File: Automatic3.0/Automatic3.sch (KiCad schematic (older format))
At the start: 56 parts, among them J1 GND VCC, J10 Line Tracker and Proximity, J11 Compass, J12 Bluetooth, J13 Encoder, J14 Bluetooth, J15 Motor, J19 Bluetooth, J2 CONN_01X01, J4 CONN_01X01, J5 CONN_01X01, J6 I/O Pins, J7 USB_B, J8 CONN_01X01, J9 I/O Pins, U1 Arduino_Mega2560_Shield, U2 Arduino_Mega2560_Shield

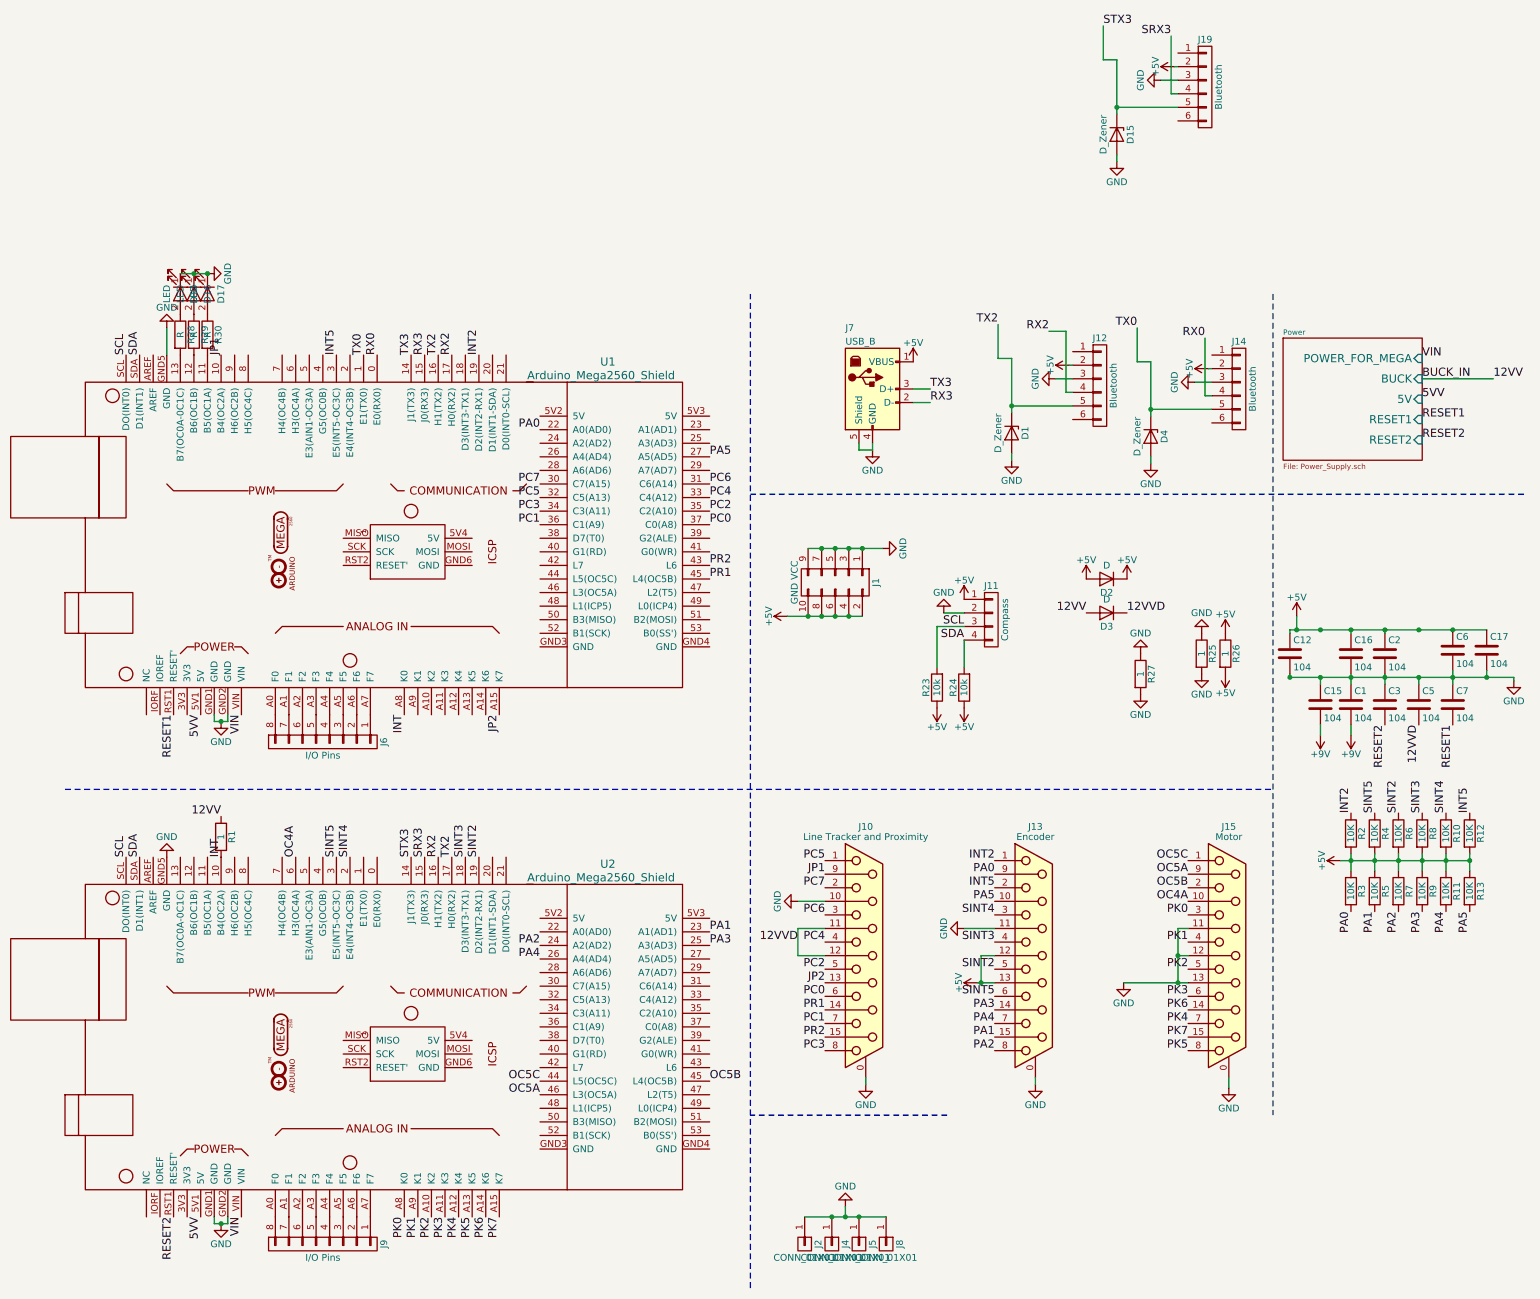
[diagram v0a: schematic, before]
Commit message: modified the automatic circuit
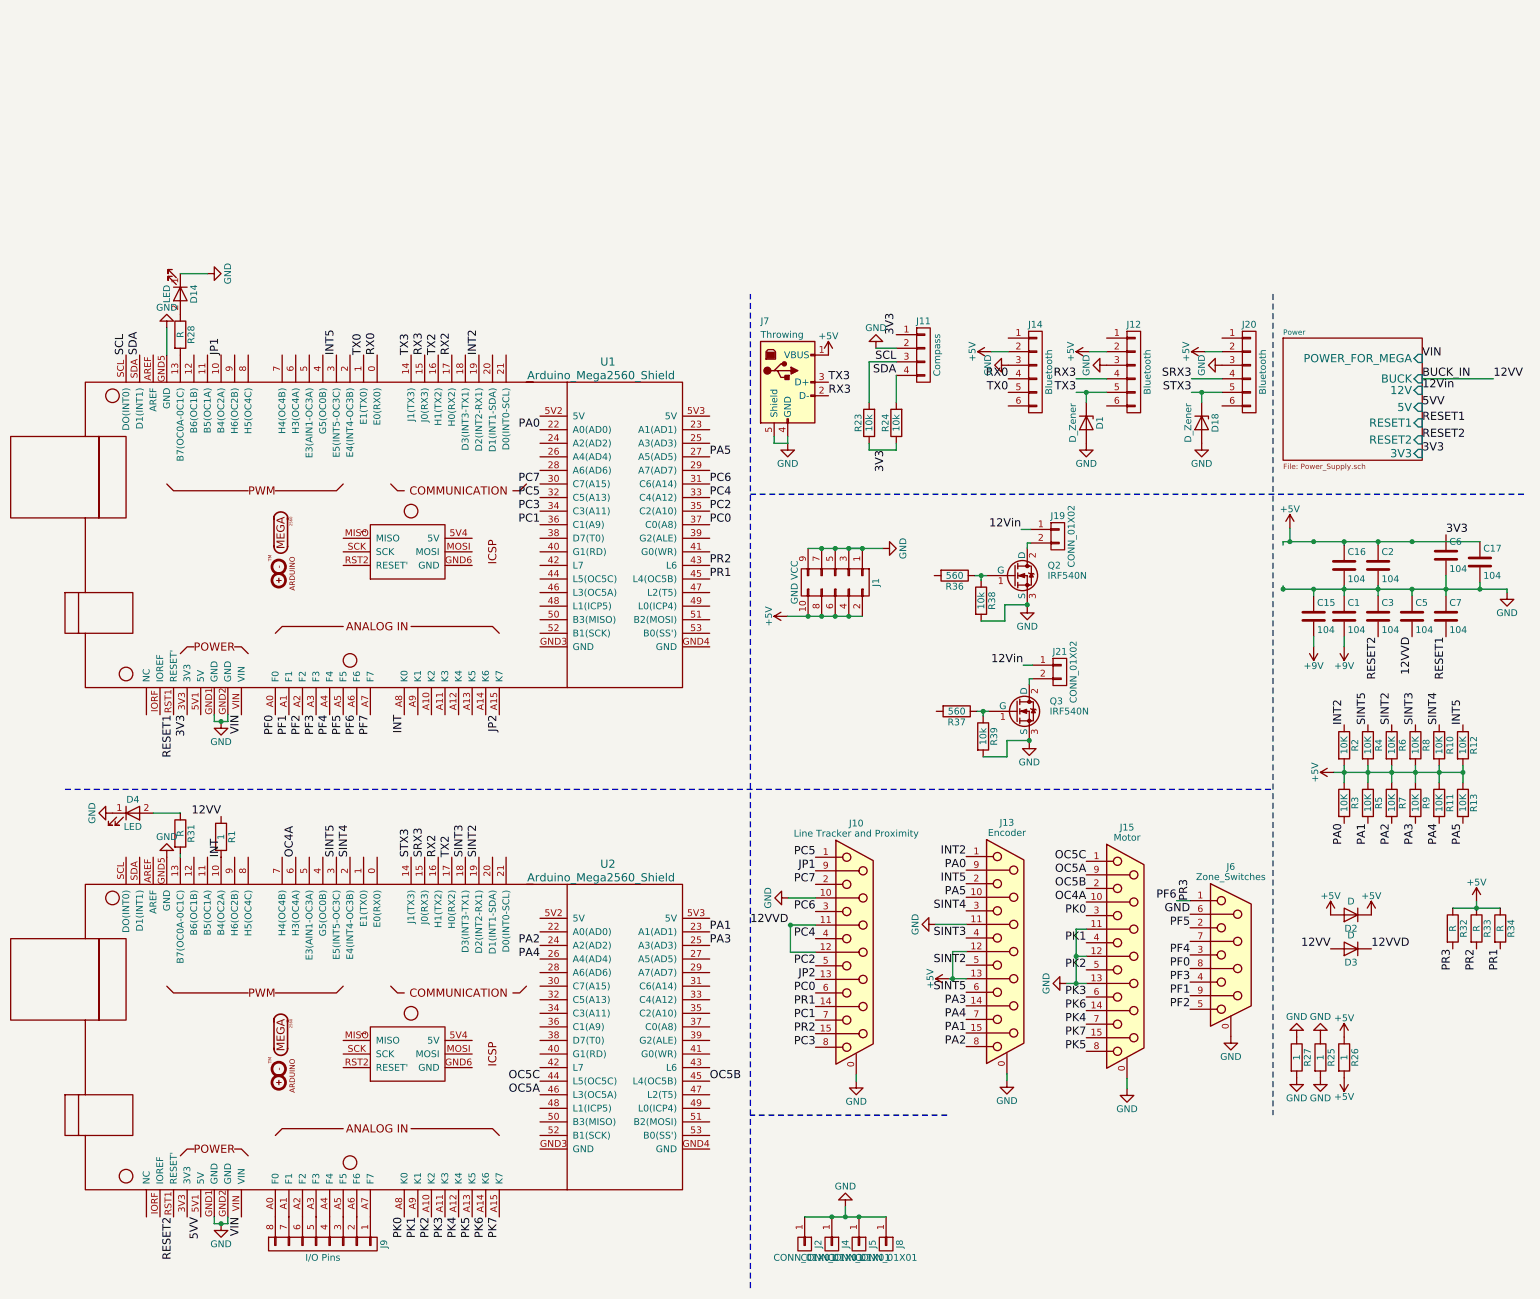
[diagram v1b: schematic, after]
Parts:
- removed C12: 104, modFiles:Capacitor_Disc_Medium, symbol C
- removed D15, D4: D_Zener, Diodes_THT:D_DO-35_SOD27_P7.62mm_Horizontal, symbol D_Zener
- removed D16, D17: LED, modFiles:LED_D3.0mm, symbol LED
- removed J19: Bluetooth, Pin_Headers:Pin_Header_Straight_1x06_Pitch2.54mm, symbol CONN_01X06
- removed J6: I/O Pins, Pin_Headers:Pin_Header_Straight_1x08_Pitch2.54mm, symbol CONN_01X08
- removed R29, R30: R, modFiles:Resistor_small, symbol R
- added D18: D_Zener, Diodes_THT:D_DO-35_SOD27_P7.62mm_Horizontal, symbol D_Zener
- added D4: LED, modFiles:LED_D3.0mm, symbol LED
- added J19, J21: CONN_01X02, modFiles:Connector_Bornier_2, symbol CONN_01X02
- added J20: Bluetooth, Pin_Headers:Pin_Header_Straight_1x06_Pitch2.54mm, symbol CONN_01X06
- added J6: Zone_Switches, modFiles:Connector_DB_9, symbol DB9_Female_MountingHoles
- added Q2, Q3: IRF540N, modFiles:Voltage_Regulators, symbol IRF540N
- added R31, R32, R33, R34: R, modFiles:Resistor_small, symbol R
- added R36, R37: 560, modFiles:Resistor_small, symbol R
- added R38, R39: 10k, modFiles:Resistor_small, symbol R
- D2, D3: footprint modFiles:Diode_Small -> modFiles:Diode_small
- J11: footprint Connectors_JST:JST_PH_B4B-PH-K_04x2.00mm_Straight -> Connectors_JST:JST_XH_B04B-XH-A_04x2.50mm_Straight
- J2, J4, J5, J8: footprint Connectors:1pin -> modFiles:1_Pin
- J7: value USB_B -> Throwing; footprint Connectors_JST:JST_PH_B4B-PH-K_04x2.00mm_Straight -> Connectors_JST:JST_XH_B04B-XH-A_04x2.50mm_Straight
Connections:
- net +5V: now also J20.2 (P2), R32.1, R33.1, R34.1; no longer C6.1, J11.1 (P1), R23.1, R24.1
- net 5VV: no longer U1.5V1 (5V)
- net GND: now also D18.2 (A), D4.1 (K), J20.3 (P3), J6.0 (PAD), J6.6, Q2.3 (S), Q3.3 (S), R38.2, R39.2
- net PR1: now also R34.2
- net PR2: now also R33.2
- net RX2: no longer J12.4 (P4)
- net RX3: now also J12.4 (P4)
- net SCL: no longer U2.SCL (DO(INT0))
- net SDA: no longer U2.SDA (D1(INT1))
- net SRX3: now also J20.4 (P4)
- net STX3: now also D18.1 (K), J20.5 (P5)
- net TX2: no longer D1.1 (K), J12.5 (P5)
- net TX3: now also D1.1 (K), J12.5 (P5)
- net 3V3: now reaches U1.3V3
- net 3V3: now also C6.1, J11.1 (P1), R23.1, R24.1
- net PF0: now reaches U1.A0 (F0)
- net PF0: now also J6.8
- net PF1: now reaches U1.A1 (F1)
- net PF1: now also J6.9
- net PF2: now reaches U1.A2 (F2)
- net PF2: now also J6.5
- net PF3: now reaches U1.A3 (F3)
- net PF3: now also J6.4
- net PF4: now reaches U1.A4 (F4)
- net PF4: now also J6.3
- net PF5: now reaches U1.A5 (F5)
- net PF5: now also J6.2
- net PF6: now reaches U1.A6 (F6)
- net PF6: now also J6.1, R32.2
- net PF7: now reaches U1.A7 (F7)
- net at U2.13 (B7(OC0A-0C1C)): now also R31.2
- new net: D4.2 (A), R31.1
- new net: Q2.1 (G), R36.1, R38.1
- new net: J19.2 (P2), Q2.2 (D)
- new net: Q3.1 (G), R37.1, R39.1
- new net: J21.2 (P2), Q3.2 (D)
- new net 12Vin: J19.1 (P1), J21.1 (P1)
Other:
- moved on the sheet: C1, C15, C16, C17, C2, C3, C5, C6, C7, D1, D2, D3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
